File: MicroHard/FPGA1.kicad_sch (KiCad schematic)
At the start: 18 parts, among them J6 FPGA_GPIO_header, U4 XC7A100T-FTG256, Y2 CB3-3C-20M000000

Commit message: VGA and Display layout
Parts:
- J6: footprint Connector_JST:JST_XH_B8B-XH-AM_1x08_P2.50mm_Vertical -> Connector_PinHeader_2.54mm:PinHeader_1x08_P2.54mm_Vertical
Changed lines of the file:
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@@
 			)
 		)
-		(property "Footprint" "Connector_JST:JST_XH_B8B-XH-AM_1x08_P2.50mm_Vertical"
+		(property "Footprint" "Connector_PinHeader_2.54mm:PinHeader_1x08_P2.54mm_Vertical"
 			(at 280.67 110.49 0)
 			(effects

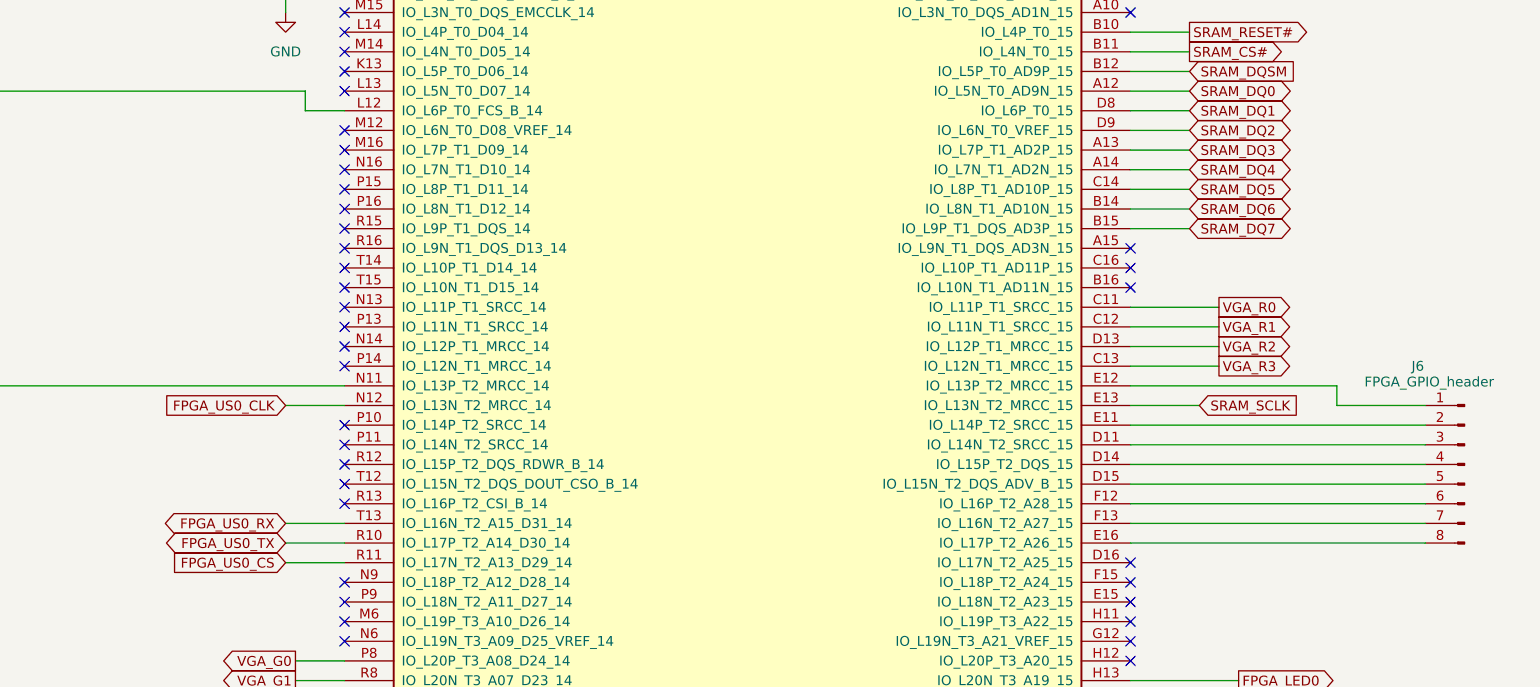
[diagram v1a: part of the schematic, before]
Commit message: finished FPGA
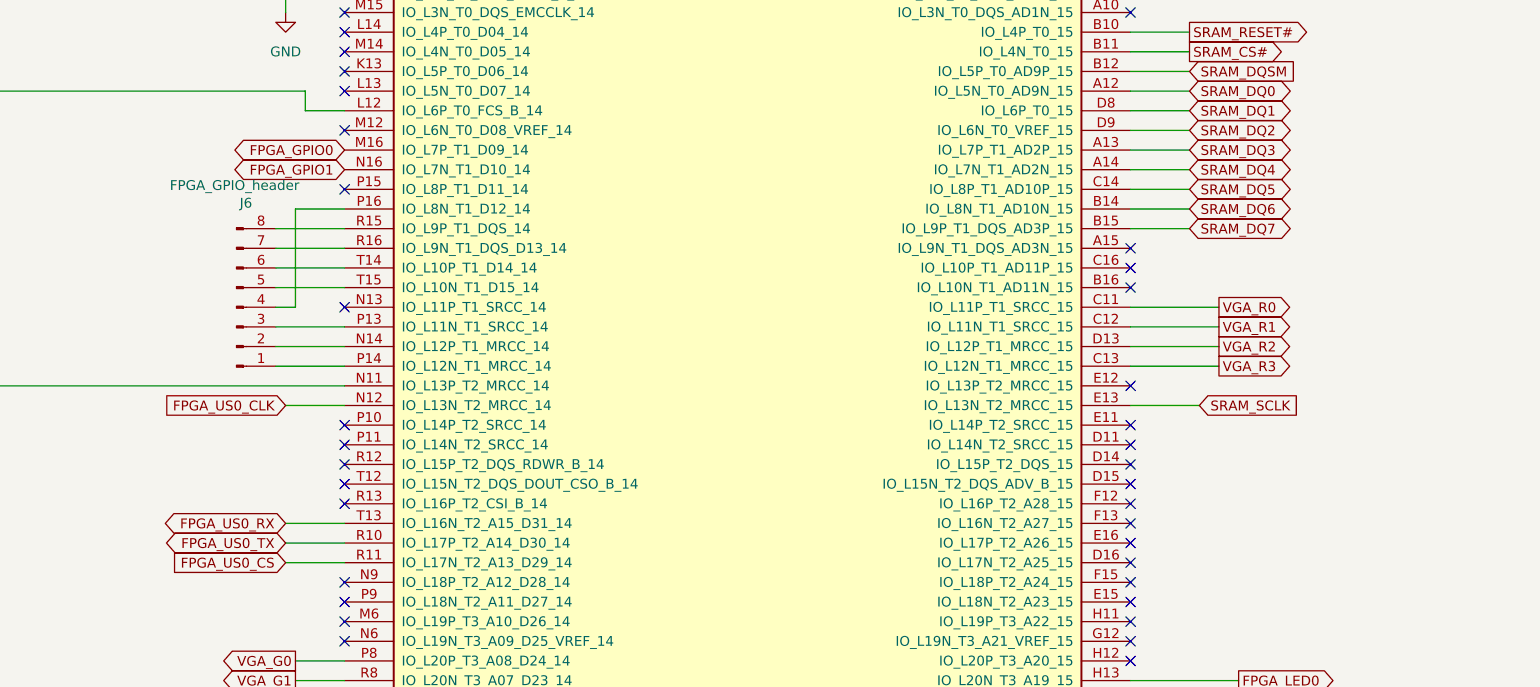
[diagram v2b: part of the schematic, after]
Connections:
- net at U4.D11 (IO_L14N_T2_SRCC_15): no longer J6.3 (Pin_3)
- net at U4.D14 (IO_L15P_T2_DQS_15): no longer J6.4 (Pin_4)
- net at U4.D15 (IO_L15N_T2_DQS_ADV_B_15): no longer J6.5 (Pin_5)
- net at U4.E11 (IO_L14P_T2_SRCC_15): no longer J6.2 (Pin_2)
- net at U4.E12 (IO_L13P_T2_MRCC_15): no longer J6.1 (Pin_1)
- net at U4.E16 (IO_L17P_T2_A26_15): no longer J6.8 (Pin_8)
- net at U4.F12 (IO_L16P_T2_A28_15): no longer J6.6 (Pin_6)
- net at U4.F13 (IO_L16N_T2_A27_15): no longer J6.7 (Pin_7)
- net FPGA_GPIO0: now reaches U4.M16 (IO_L7P_T1_D09_14)
- net at U4.N14 (IO_L12P_T1_MRCC_14): now also J6.2 (Pin_2)
- net FPGA_GPIO1: now reaches U4.N16 (IO_L7N_T1_D10_14)
- net at U4.P13 (IO_L11N_T1_SRCC_14): now also J6.3 (Pin_3)
- net at U4.P14 (IO_L12N_T1_MRCC_14): now also J6.1 (Pin_1)
- net at U4.P16 (IO_L8N_T1_D12_14): now also J6.4 (Pin_4)
- net at U4.R15 (IO_L9P_T1_DQS_14): now also J6.8 (Pin_8)
- net at U4.R16 (IO_L9N_T1_DQS_D13_14): now also J6.7 (Pin_7)
- net at U4.T14 (IO_L10P_T1_D14_14): now also J6.6 (Pin_6)
- net at U4.T15 (IO_L10N_T1_D15_14): now also J6.5 (Pin_5)
- no-connect marks 50 -> 48
